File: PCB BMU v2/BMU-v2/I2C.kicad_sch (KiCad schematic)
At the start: 33 parts, among them J2 RJ45_Shielded, J4 RJ45_Shielded, U6 TCA9535PWR, U8 ISO1540DR

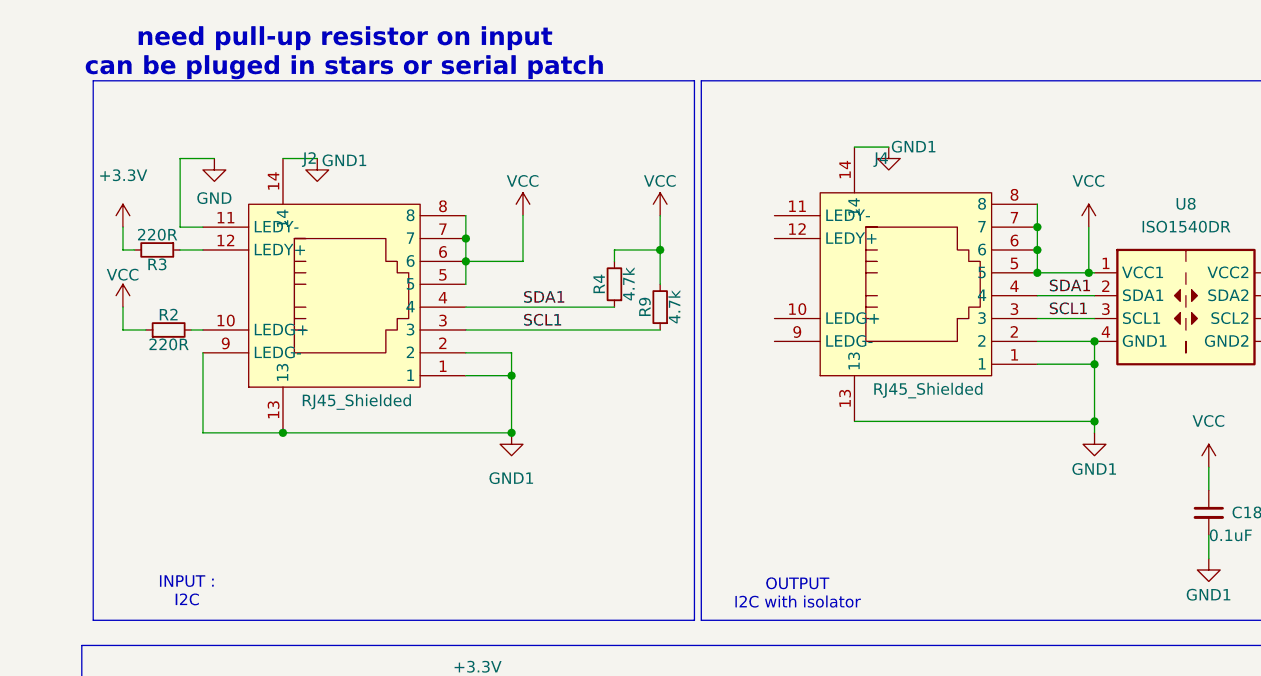
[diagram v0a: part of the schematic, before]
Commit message: update PCB
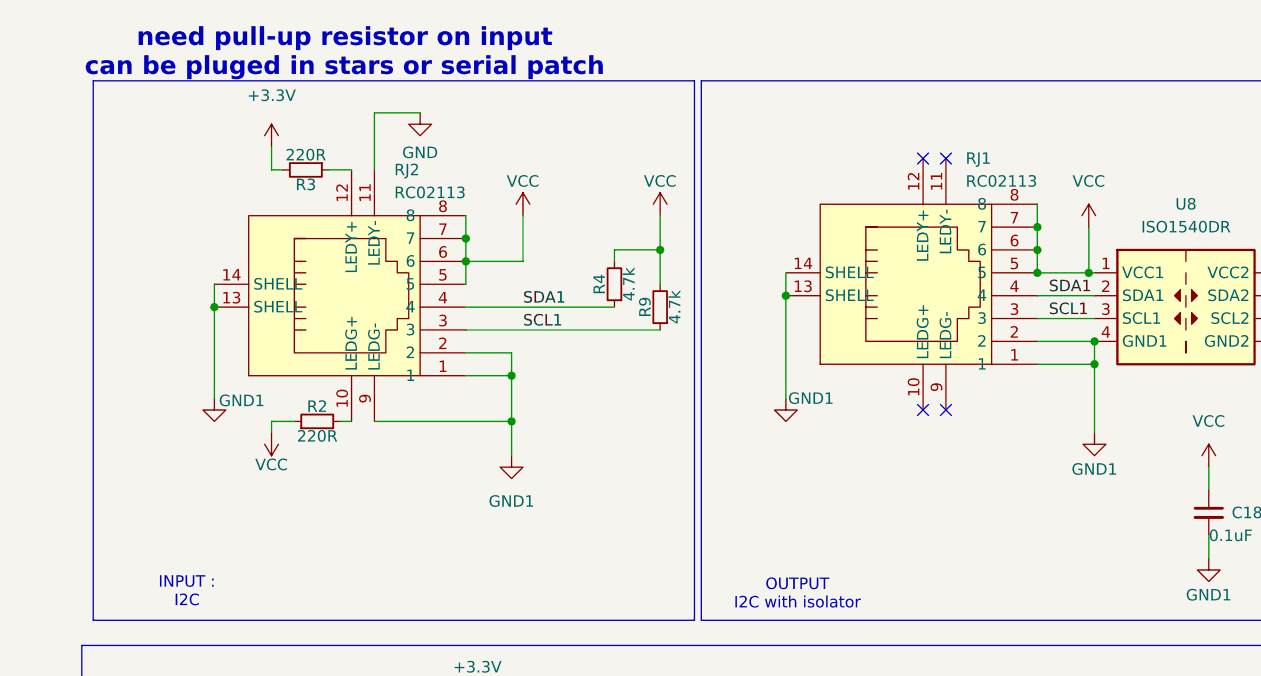
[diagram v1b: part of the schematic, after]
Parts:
- removed J2, J4: RJ45_Shielded, easyeda2kicad:RJ45-TH_RC02535, symbol easyeda2kicad:RC01061
- added RJ1, RJ2: RC02113, easyeda2kicad:RJ45-TH_RC02113, symbol easyeda2kicad:RC02113
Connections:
- net GND: now also RJ2.11 (LEDY-)
- net GND1: now also RJ1.1, RJ1.13 (SHELL), RJ1.14 (SHELL), RJ1.2, RJ2.1, RJ2.13 (SHELL), RJ2.14 (SHELL), RJ2.2, RJ2.9 (LEDG-)
- net SCL1: now also RJ1.3, RJ2.3
- net SDA1: now also RJ1.4, RJ2.4
- net VCC: now also RJ1.5, RJ1.6, RJ1.7, RJ1.8, RJ2.5, RJ2.6, RJ2.7, RJ2.8
- net at R2.2: now also RJ2.10 (LEDG+)
- net at R3.1: now also RJ2.12 (LEDY+)
- no-connect marks 0 -> 4
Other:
- moved on the sheet: R2, R3
